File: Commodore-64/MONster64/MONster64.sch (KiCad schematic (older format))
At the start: 90 parts, among them J1 USB Power, J10 USB_B_Micro, J11 Hirose_DM3D-SF, J12 Conn_01x20, J13 RJ45_Amphenol_RJMG1BD3B8K1ANR, J2 CLOCK_JUMPER, J3 3v3, J4 4pin Expansion, J5 Conn_01x20, J6 GND, J7 3v3, J8 GND, J9 SWD, Q1 BC846BLT1G, SW1 Reset, SW2 Menu, SW3 Special, U1 STM32H753VIT6, U2 TXS0108EQPWRQ1, U3 W25M02GWZEIG, U4 DP83822IFRHB, X1 DSC1001, Y1 Crystal

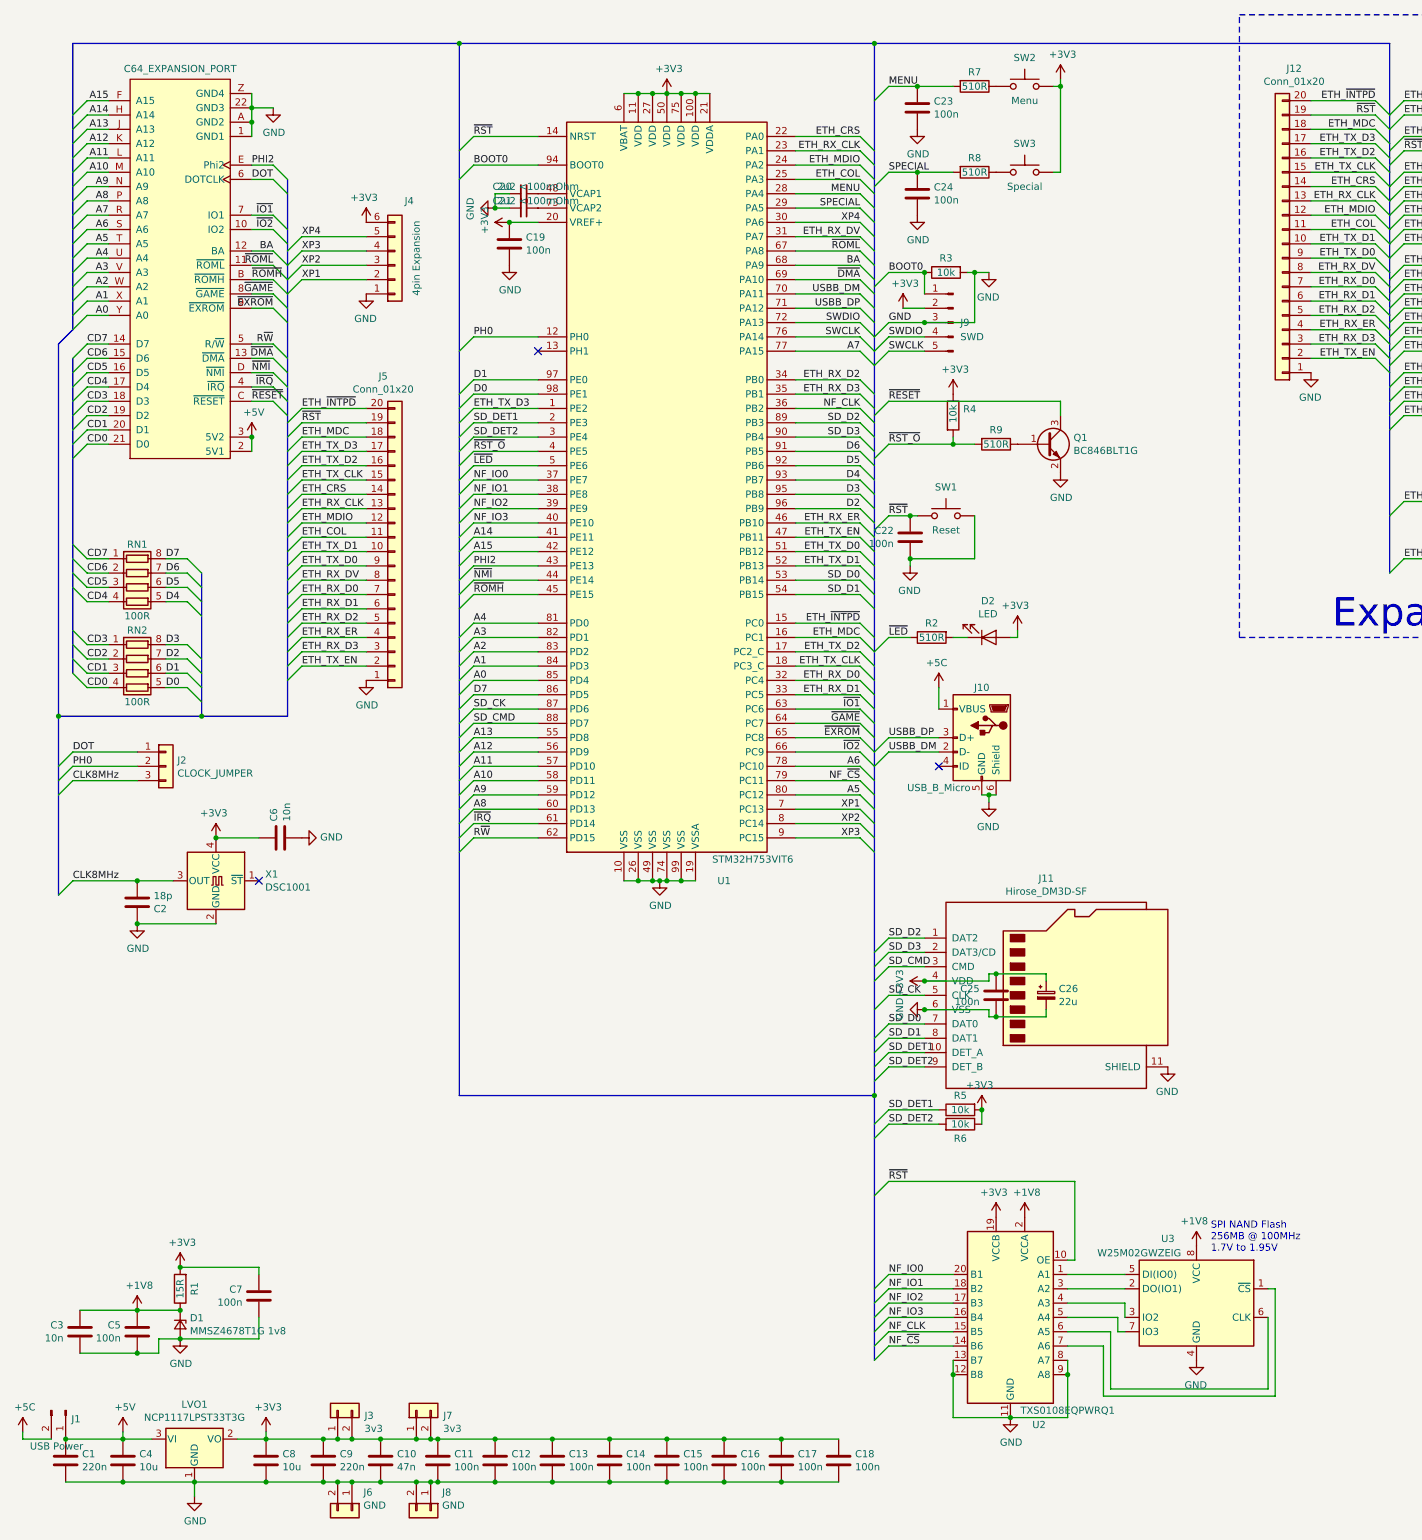
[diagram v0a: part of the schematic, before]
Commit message: Changed over for 1v8 operation
- Level Translated DOTCLK for OSC_IN
- JTAG header requires 5v instead of 3v3 to power board
- NAND Flash memory directly connected instead of through a TXS0108
- Dual regulator to streamline power domains.
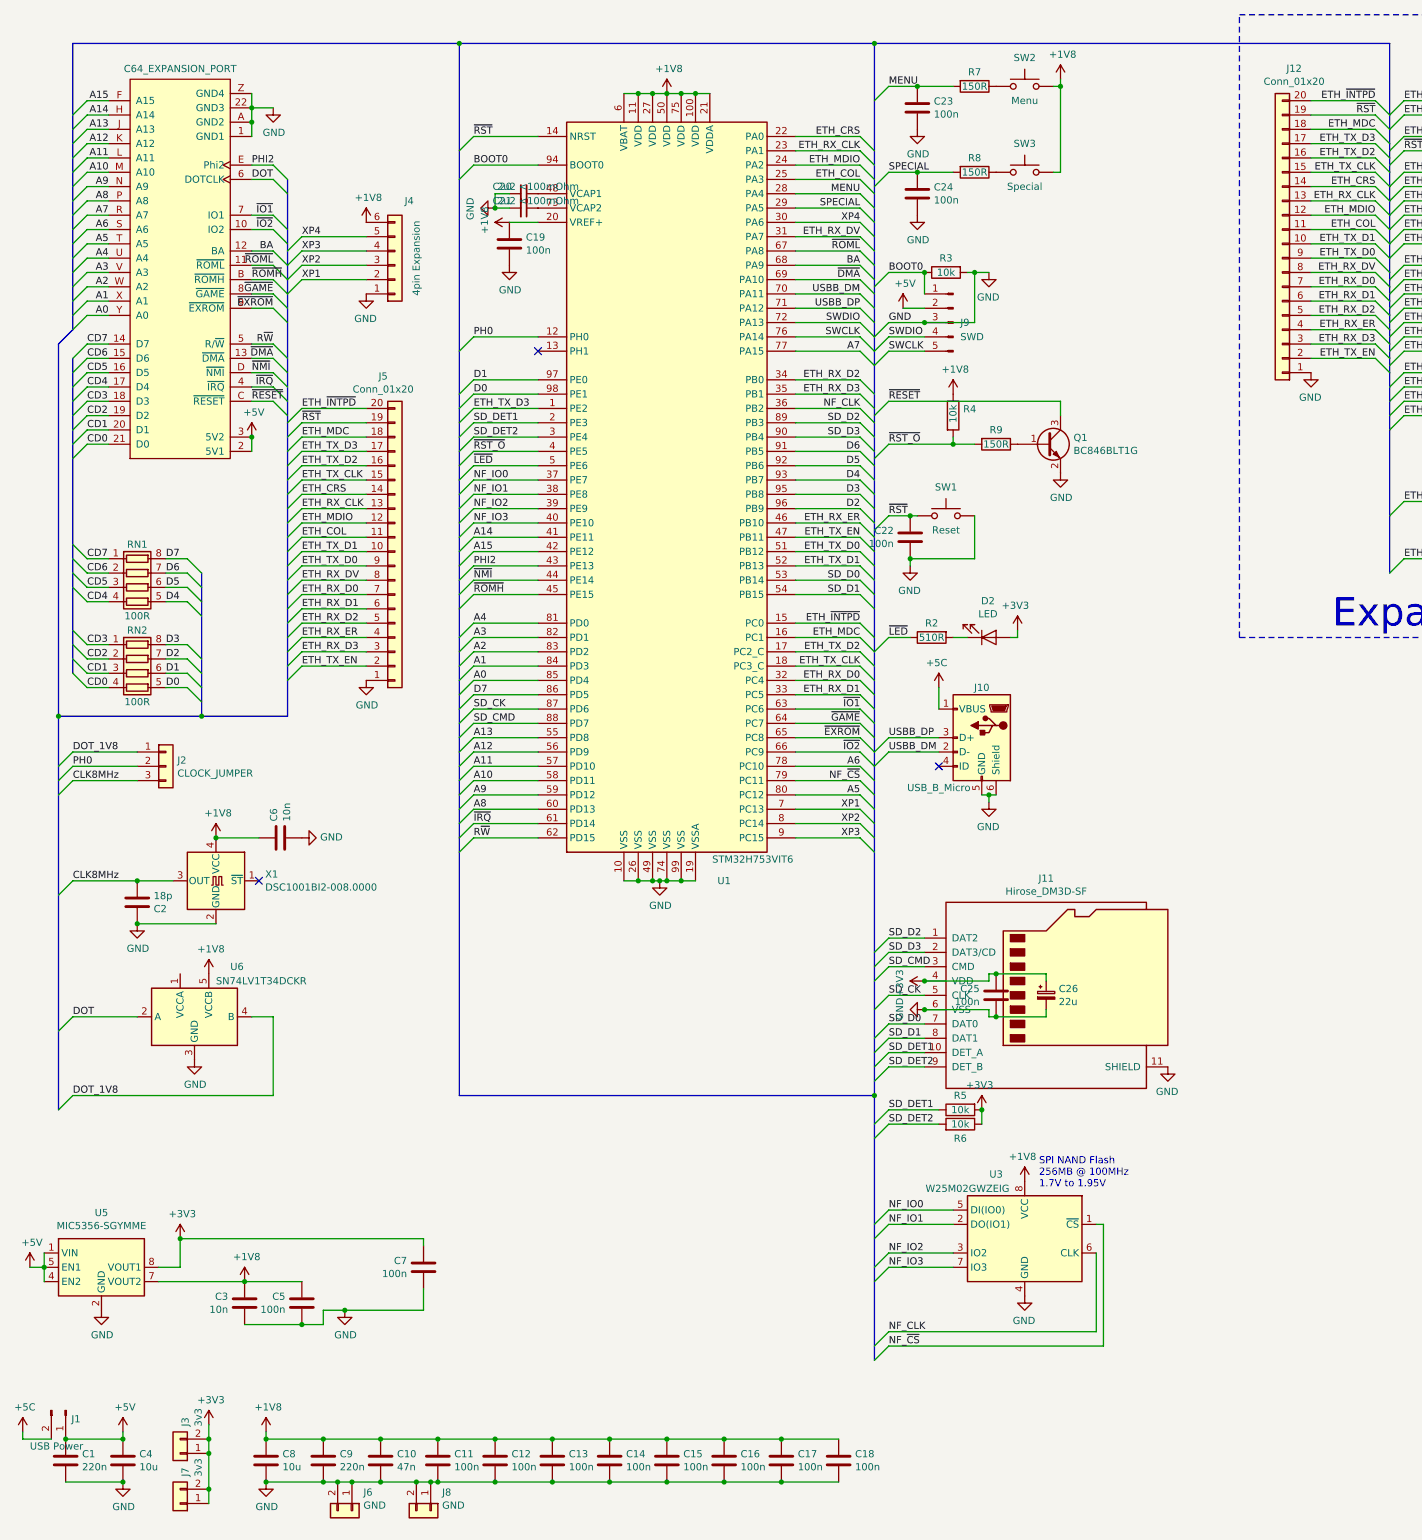
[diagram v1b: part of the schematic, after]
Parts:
- removed D1: MMSZ4678T1G 1v8, Diode_SMD:D_SOD-123, symbol Device:D_Zener_Small
- removed LVO1: NCP1117LPST33T3G, Package_TO_SOT_SMD:SOT-223-3_TabPin2, symbol Regulator_Linear:AMS1117-3.3
- removed R1: 15R, Resistor_SMD:R_0805_2012Metric_Pad1.15x1.40mm_HandSolder, symbol Device:R
- removed U2: TXS0108EQPWRQ1, Package_SO:TSSOP-20_4.4x6.5mm_P0.65mm, symbol Logic_LevelTranslator:TXS0108EPW
- added U5: MIC5356-SGYMME, Package_SO:MSOP-8-1EP_3x3mm_P0.65mm_EP2.5x3mm_Mask1.73x2.36mm_ThermalVias, symbol Regulator_Linear:MIC5356-SGYMME
- added U6: SN74LV1T34DCKR, Package_TO_SOT_SMD:SOT-353_SC-70-5, symbol Logic_LevelTranslator:SN74AUP1T34DCK
- R7, R8, R9: value 510R -> 150R
- RN1, RN2: footprint Resistor_SMD:R_Array_Convex_4x1206 -> Resistor_SMD:R_Array_Concave_4x0603
- X1: value DSC1001 -> DSC1001BI2-008.0000
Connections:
- net +1V8: now also C10.1, C11.1, C12.1, C13.1, C14.1, C15.1, C16.1, C17.1, C18.1, C19.1, C6.1, C8.1, C9.1, J4.6 (Pin_6), R4.1, SW2.1, SW3.1, U1.100 (VDD), U1.11 (VDD), U1.20 (VREF+), U1.21 (VDDA), U1.27 (VDD), U1.50 (VDD), U1.6 (VBAT), U1.75 (VDD), X1.4 (VCC), U5.7 (VOUT2), U6.5 (VCCB)
- net +3V3: now also U5.8 (VOUT1); no longer C10.1, C11.1, C12.1, C13.1, C14.1, C15.1, C16.1, C17.1, C18.1, C19.1, C6.1, C8.1, C9.1, J4.6 (Pin_6), J9.2 (Pin_2), R4.1, SW2.1, SW3.1, U1.100 (VDD), U1.11 (VDD), U1.20 (VREF+), U1.21 (VDDA), U1.27 (VDD), U1.50 (VDD), U1.6 (VBAT), U1.75 (VDD), X1.4 (VCC)
- net +5V: now also J9.2 (Pin_2), U5.1 (VIN), U5.4 (EN2), U5.5 (EN1)
- net DOT: now also U6.2 (A); no longer J2.1 (Pin_1)
- net GND: now also U5.2 (GND), U5.9 (GND), U6.3 (GND)
- net NF_CLK: now also U3.6 (CLK)
- net NF_IO0: now also U3.5 (DI(IO0))
- net NF_IO1: now also U3.2 (DO(IO1))
- net NF_IO2: now also U3.3 (IO2)
- net NF_IO3: now also U3.7 (IO3)
- net NF_~CS: now also U3.1 (~CS)
- new net DOT_1V8: J2.1 (Pin_1), U6.4 (B)
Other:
- moved on the sheet: C3, C5, C7, J3, J7, U3

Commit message: Revert to 3v3
Still need to translate DOTclk
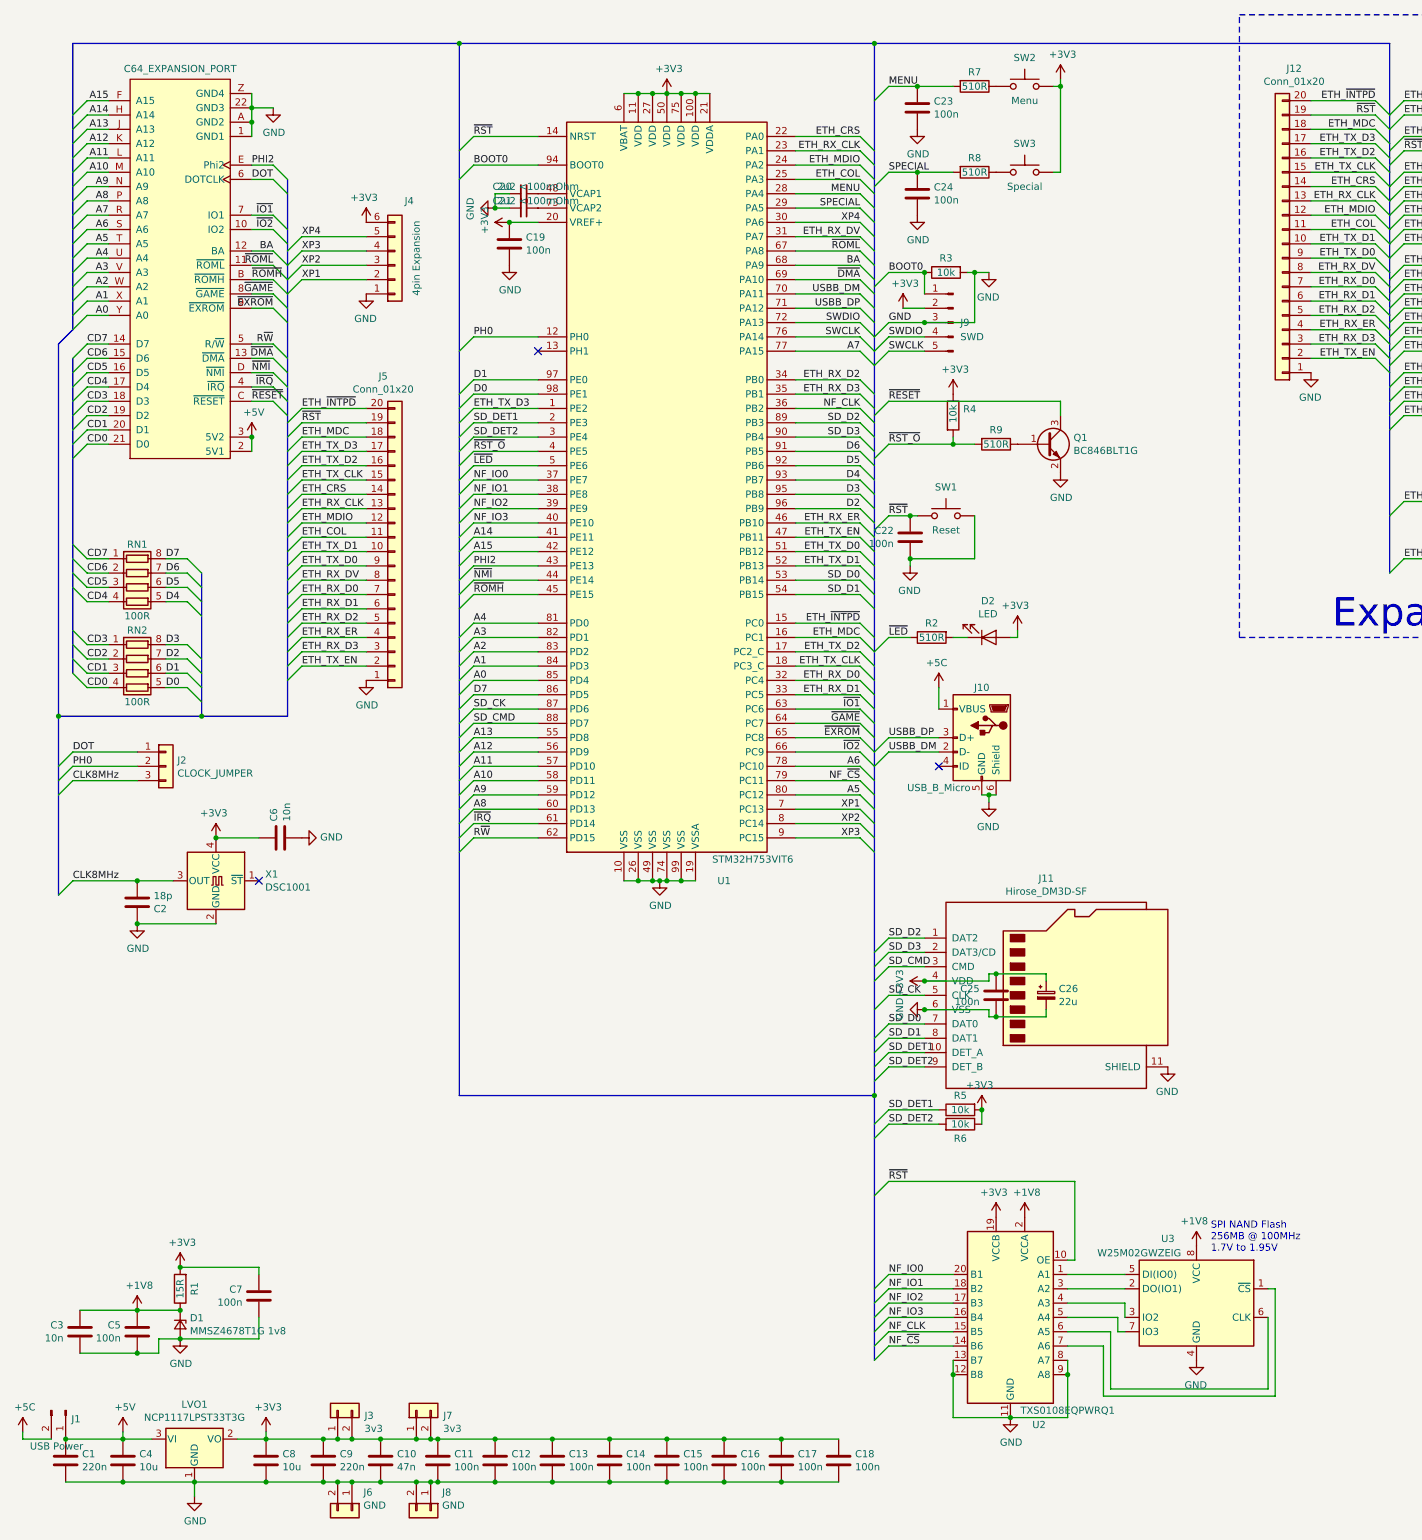
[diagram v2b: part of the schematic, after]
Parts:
- removed U5: MIC5356-SGYMME, Package_SO:MSOP-8-1EP_3x3mm_P0.65mm_EP2.5x3mm_Mask1.73x2.36mm_ThermalVias, symbol Regulator_Linear:MIC5356-SGYMME
- removed U6: SN74LV1T34DCKR, Package_TO_SOT_SMD:SOT-353_SC-70-5, symbol Logic_LevelTranslator:SN74AUP1T34DCK
- added D1: MMSZ4678T1G 1v8, Diode_SMD:D_SOD-123, symbol Device:D_Zener_Small
- added LVO1: NCP1117LPST33T3G, Package_TO_SOT_SMD:SOT-223-3_TabPin2, symbol Regulator_Linear:AMS1117-3.3
- added R1: 15R, Resistor_SMD:R_0805_2012Metric_Pad1.15x1.40mm_HandSolder, symbol Device:R
- added U2: TXS0108EQPWRQ1, Package_SO:TSSOP-20_4.4x6.5mm_P0.65mm, symbol Logic_LevelTranslator:TXS0108EPW
- R7, R8, R9: value 150R -> 510R
- RN1, RN2: footprint Resistor_SMD:R_Array_Concave_4x0603 -> Resistor_SMD:R_Array_Convex_4x1206
- X1: value DSC1001BI2-008.0000 -> DSC1001
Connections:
- net DOT_1V8 is gone; now on net DOT: J2.1 (Pin_1)
- net +1V8: now also D1.1 (K), R1.1, U2.2 (VCCA); no longer C10.1, C11.1, C12.1, C13.1, C14.1, C15.1, C16.1, C17.1, C18.1, C19.1, C6.1, C8.1, C9.1, J4.6 (Pin_6), R4.1, SW2.1, SW3.1, U1.100 (VDD), U1.11 (VDD), U1.20 (VREF+), U1.21 (VDDA), U1.27 (VDD), U1.50 (VDD), U1.6 (VBAT), U1.75 (VDD), X1.4 (VCC)
- net +3V3: now also C10.1, C11.1, C12.1, C13.1, C14.1, C15.1, C16.1, C17.1, C18.1, C19.1, C6.1, C8.1, C9.1, J4.6 (Pin_6), J9.2 (Pin_2), R4.1, SW2.1, SW3.1, U1.100 (VDD), U1.11 (VDD), U1.20 (VREF+), U1.21 (VDDA), U1.27 (VDD), U1.50 (VDD), U1.6 (VBAT), U1.75 (VDD), X1.4 (VCC), LVO1.2 (VO), R1.2, U2.19 (VCCB)
- net +5V: now also LVO1.3 (VI); no longer J9.2 (Pin_2)
- net GND: now also D1.2 (A), LVO1.1 (GND), U2.11 (GND), U2.12 (B8), U2.13 (B7), U2.8 (A7), U2.9 (A8)
- net NF_CLK: now also U2.15 (B5); no longer U3.6 (CLK)
- net NF_IO0: now also U2.20 (B1); no longer U3.5 (DI(IO0))
- net NF_IO1: now also U2.18 (B2); no longer U3.2 (DO(IO1))
- net NF_IO2: now also U2.17 (B3); no longer U3.3 (IO2)
- net NF_IO3: now also U2.16 (B4); no longer U3.7 (IO3)
- net NF_~CS: now also U2.14 (B6); no longer U3.1 (~CS)
- net ~RST: now also U2.10 (OE)
- new net: U2.7 (A6), U3.1 (~CS)
- new net: U2.3 (A2), U3.2 (DO(IO1))
- new net: U2.4 (A3), U3.3 (IO2)
- new net: U2.1 (A1), U3.5 (DI(IO0))
- new net: U2.6 (A5), U3.6 (CLK)
- new net: U2.5 (A4), U3.7 (IO3)
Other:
- moved on the sheet: C3, C5, C7, J3, J7, U3
